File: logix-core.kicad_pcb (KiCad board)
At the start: 6 copper layers, 76 parts, among them J1 QSH-030-01-X-D-A-XX, J2 QSH-030-01-X-D-A-XX, J3 878321420, U1 XC7A15T-CSG325, U1 XC7A15T-FTG256, U2 MP5470GL-0000-P, U3 TPUSBLC6-4SC6, U4 FT230XQ, U5 MX25L3233FZN, U6 XC7A15T-CSG325, U8 MT41K256M16TW-107:P

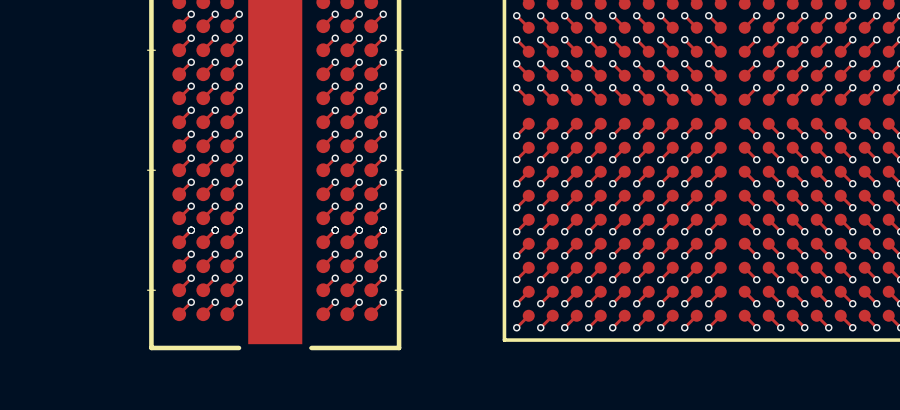
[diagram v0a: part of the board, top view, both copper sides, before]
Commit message: working for ddr3 pcb part 2
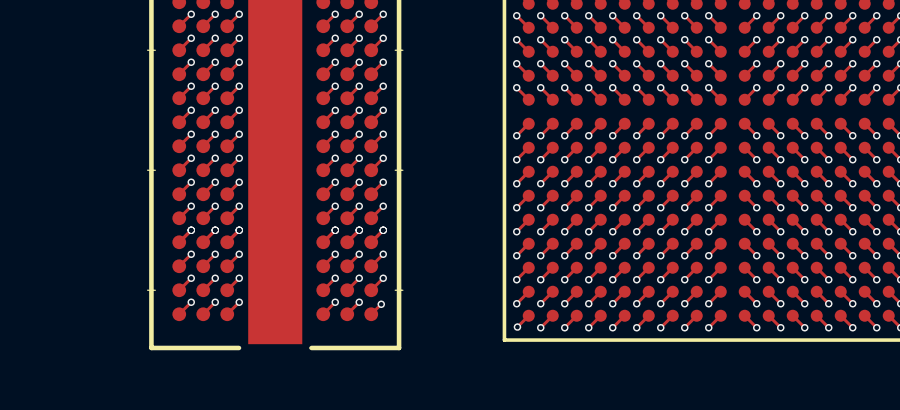
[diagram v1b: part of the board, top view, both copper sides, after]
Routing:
- net /DDR3_ADDR6: track 2.46 -> 15.7 mm
- net /DDR3_ADDR14: track 6.79 -> 19.9 mm
- net /DDR3_ADDR11: track 7.19 -> 20.2 mm
- net /DDR3_ADDR4: track 2.46 -> 14.7 mm
- net /DDR3_ADDR1: track 7.59 -> 19.5 mm
- net /DDR3_BLOCK_ADDR1: track 3.03 -> 14.1 mm
- net /DDR3/ZQ: track 1.89 -> 12.9 mm
- net /DDR3_ADDR10: track 5.78 -> 16.6 mm
- net /DDR3_ADDR8: track 6.88 -> 16.0 mm
- net GND: track 80.7 -> 75.4 mm
- net /DDR3_ADDR12: track 8.57 -> 13.5 mm
